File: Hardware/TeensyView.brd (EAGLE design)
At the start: 35.6 x 17.8 mm, 23 parts, among them J1 DNP, J2 DNP

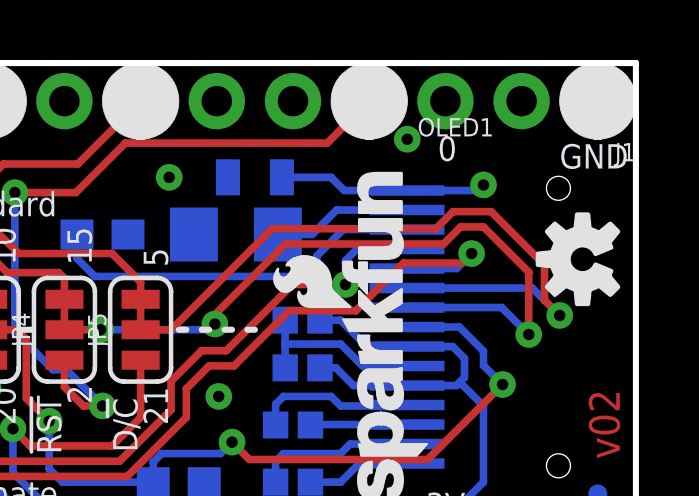
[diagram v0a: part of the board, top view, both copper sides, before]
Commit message: worked through checklist and updated some parts, moved TP
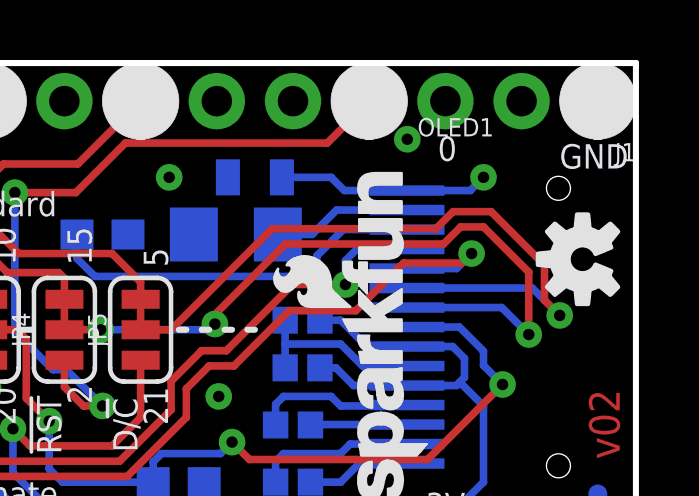
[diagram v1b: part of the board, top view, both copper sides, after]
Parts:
- C6: value 4.7UF -> 4.7uF
- OLED1: value OLED128X64SIDEREAR-MOUNT -> 32x128 OLED
- R1: value 820k -> 390k
- moved TP1 0.25 mm to (30.5, 14.0)
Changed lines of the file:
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@@
 <grid distance="0.05" unitdist="inch" unit="inch" style="lines" multiple="1" display="yes" altdistance="0.005" altunitdist="inch" altunit="inch"/>
 <layers>
-<layer number="1" name="Top" color="4" fill="1" visible="yes" active="yes"/>
+<layer number="1" name="Top" color="4" fill="1" visible="no" active="yes"/>
 <layer number="2" name="Route2" color="1" fill="3" visible="no" active="no"/>
 <layer number="3" name="Route3" color="4" fill="3" visible="no" active="no"/>
@@
 <layer number="19" name="Unrouted" color="6" fill="1" visible="yes" active="yes"/>
 <layer number="20" name="Dimension" color="15" fill="1" visible="yes" active="yes"/>
-<layer number="21" name="tPlace" color="16" fill="1" visible="yes" active="yes"/>
+<layer number="21" name="tPlace" color="16" fill="1" visible="no" active="yes"/>
 <layer number="22" name="bPlace" color="14" fill="1" visible="yes" active="yes"/>
-<layer number="23" name="tOrigins" color="15" fill="1" visible="no" active="yes"/>
-<layer number="24" name="bOrigins" color="15" fill="1" visible="no" active="yes"/>
+<layer number="23" name="tOrigins" color="15" fill="1" visible="yes" active="yes"/>
+<layer number="24" name="bOrigins" color="15" fill="1" visible="yes" active="yes"/>
 <layer number="25" name="tNames" color="7" fill="1" visible="no" active="yes"/>
 <layer number="26" name="bNames" color="7" fill="1" visible="no" active="yes"/>
@@
 <layer number="43" name="vRestrict" color="2" fill="10" visible="no" active="yes"/>
 <layer number="44" name="Drills" color="7" fill="1" visible="no" active="yes"/>
-<layer number="45" name="Holes" color="7" fill="1" visible="no" active="yes"/>
+<layer number="45" name="Holes" color="7" fill="1" visible="yes" active="yes"/>
 <layer number="46" name="Milling" color="3" fill="1" visible="no" active="yes"/>
 <layer number="47" name="Measures" color="7" fill="1" visible="no" active="yes"/>
@@
 <layer number="49" name="Reference" color="7" fill="1" visible="no" active="yes"/>
 <layer number="50" name="dxf" color="7" fill="1" visible="no" active="no"/>
-<layer number="51" name="tDocu" color="6" fill="1" visible="no" active="yes"/>
+<layer number="51" name="tDocu" color="6" fill="1" visible="yes" active="yes"/>
 <layer number="52" name="bDocu" color="7" fill="1" visible="no" active="yes"/>
 <layer number="53" name="tGND_GNDA" color="7" fill="9" visible="no" active="no"/>
@@
 <element name="LOGO2" library="SparkFun-Aesthetics" package="OSHW-LOGO-S" value="OSHW-LOGOS" x="33.782" y="11.2395" rot="R90"/>
 <element name="LOGO3" library="SparkFun-Aesthetics" package="SFE_LOGO_NAME_FLAME_.1" value="SFE_LOGO_NAME_FLAME.1_INCH" x="28.6940625" y="2.7860625" rot="R90"/>
-<element name="OLED1" library="TeensyViewDev" package="OLED-UG-2832TSWGG01-REAR" value="OLED128X64SIDEREAR-MOUNT" x="27.178" y="14.605"/>
+<element name="OLED1" library="TeensyViewDev" package="OLED-UG-2832TSWGG01-REAR" value="32x128 OLED" x="27.178" y="14.605">
+<attribute name="VALUE" value="32x128 OLED" x="27.178" y="14.605" size="1.778" layer="27" display="off"/>
+<attribute name="PROD_ID" value="LCD-13577" x="27.178" y="14.605" size="1.778" layer="27" display="off"/>
+</element>
 <element name="C1" library="SparkFun-Capacitors" package="0402" value="1.0uF" x="24.4475" y="7.62" rot="MR0">
 <attribute name="PROD_ID" value="CAP-12417" x="24.4475" y="7.62" size="1.778" layer="28" font="vector" ratio="15" rot="MR0" display="off"/>
@@
 <attribute name="PROD_ID" value="CAP-11624" x="22.86" y="13.97" size="1.778" layer="28" font="vector" ratio="15" rot="MR0" display="off"/>
 </element>
-<element name="C6" library="SparkFun-Capacitors" package="1206" value="4.7UF" x="22.225" y="12.065" rot="MR0">
+<element name="C6" library="SparkFun-Capacitors" package="1206" value="4.7uF" x="22.225" y="12.065" rot="MR0">
 <attribute name="PROD_ID" value="CAP-10300" x="22.225" y="12.065" size="1.778" layer="28" rot="MR0" display="off"/>
+<attribute name="VALUE" value="4.7uF" x="22.225" y="12.065" size="1.778" layer="28" rot="MR0" display="off"/>
 </element>
-<element name="R1" library="SparkFun-Resistors" package="0603" value="820k" x="17.78" y="12.065" rot="MR0">
-<attribute name="PROD_ID" value="RES-13247" x="17.78" y="12.065" size="1.778" layer="28" font="vector" ratio="15" rot="MR0" display="off"/>
+<element name="R1" library="SparkFun-Resistors" package="0603" value="390k" x="17.78" y="12.065" rot="MR0">
+<attribute name="PROD_ID" value="RES-12024" x="17.78" y="12.065" size="1.778" layer="28" font="vector" ratio="15" rot="MR0" display="off"/>
 </element>
 <element name="JP1" library="SparkFun-Jumpers" package="SMT-JUMPER_3_1-NC_TRACE_SILK" value="JUMPER-SMT_3_1-NC_TRACE_SILK" x="13.97" y="8.89" rot="R90"/>
@@
 <element name="JP4" library="SparkFun-Jumpers" package="SMT-JUMPER_3_1-NC_TRACE_SILK" value="JUMPER-SMT_3_1-NC_TRACE_SILK" x="16.51" y="8.89" rot="R90"/>
 <element name="JP5" library="SparkFun-Jumpers" package="SMT-JUMPER_3_1-NC_TRACE_SILK" value="JUMPER-SMT_3_1-NC_TRACE_SILK" x="19.05" y="8.89" rot="R90"/>
-<element name="TP1" library="SparkFun-Connectors" package="TP_15TH" value="TEST-POINTTP_15TH_THRU" x="30.48" y="13.716" rot="MR0"/>
+<element name="TP1" library="SparkFun-Connectors" package="TP_15TH" value="TEST-POINTTP_15TH_THRU" x="30.48" y="13.97" rot="MR0"/>
 </elements>
 <signals>
@@
 <wire x1="25.4" y1="13.97" x2="23.76" y2="13.97" width="0.254" layer="16"/>
 <contactref element="TP1" pad="P$1"/>
-<wire x1="27.928" y1="13.53" x2="30.294" y2="13.53" width="0.254" layer="16"/>
-<wire x1="30.294" y1="13.53" x2="30.48" y2="13.716" width="0.254" layer="16"/>
+<wire x1="27.928" y1="13.53" x2="30.04" y2="13.53" width="0.254" layer="16"/>
+<wire x1="30.04" y1="13.53" x2="30.48" y2="13.97" width="0.254" layer="16"/>
 </signal>
 <signal name="!CS">
